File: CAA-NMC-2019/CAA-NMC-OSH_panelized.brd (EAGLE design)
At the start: 115.2 x 110.2 mm, 18 parts, among them IC1 ATTINY85-20SU, J1 M20-9980346

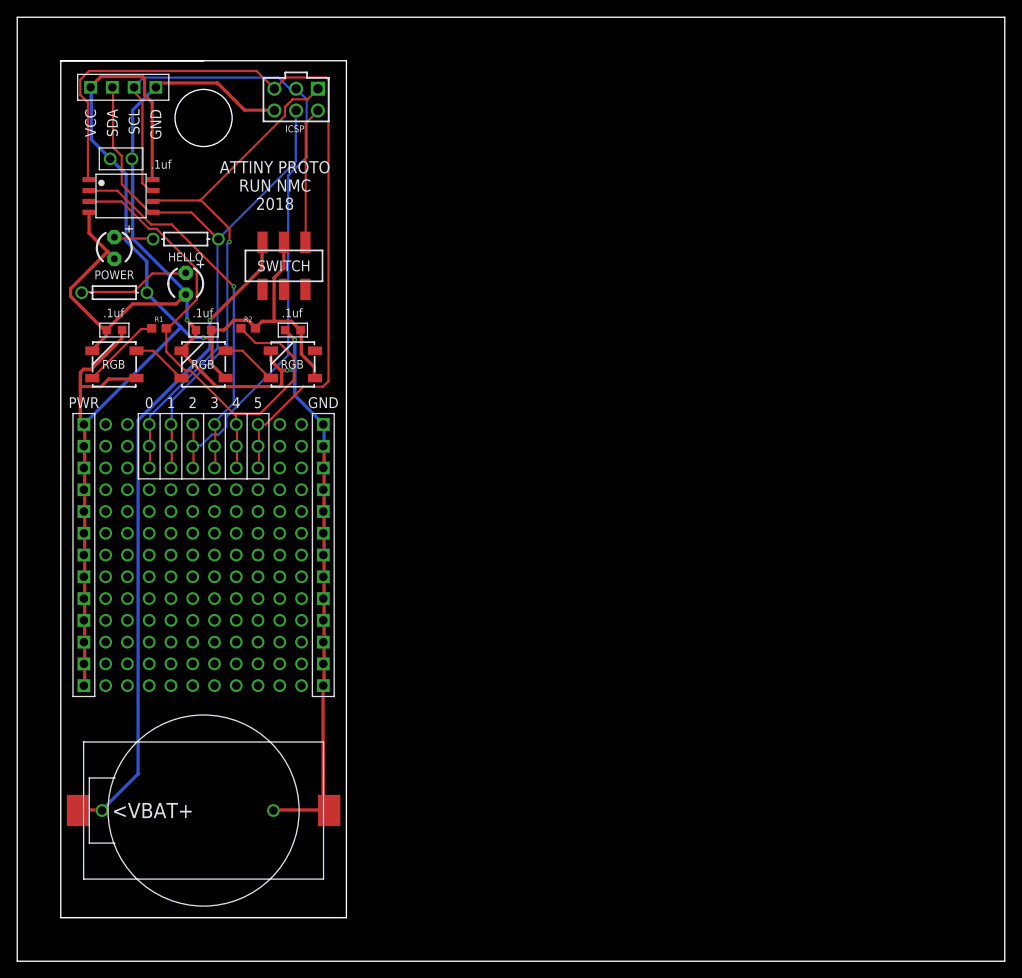
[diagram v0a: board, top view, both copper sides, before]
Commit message: Finalized file for OSH
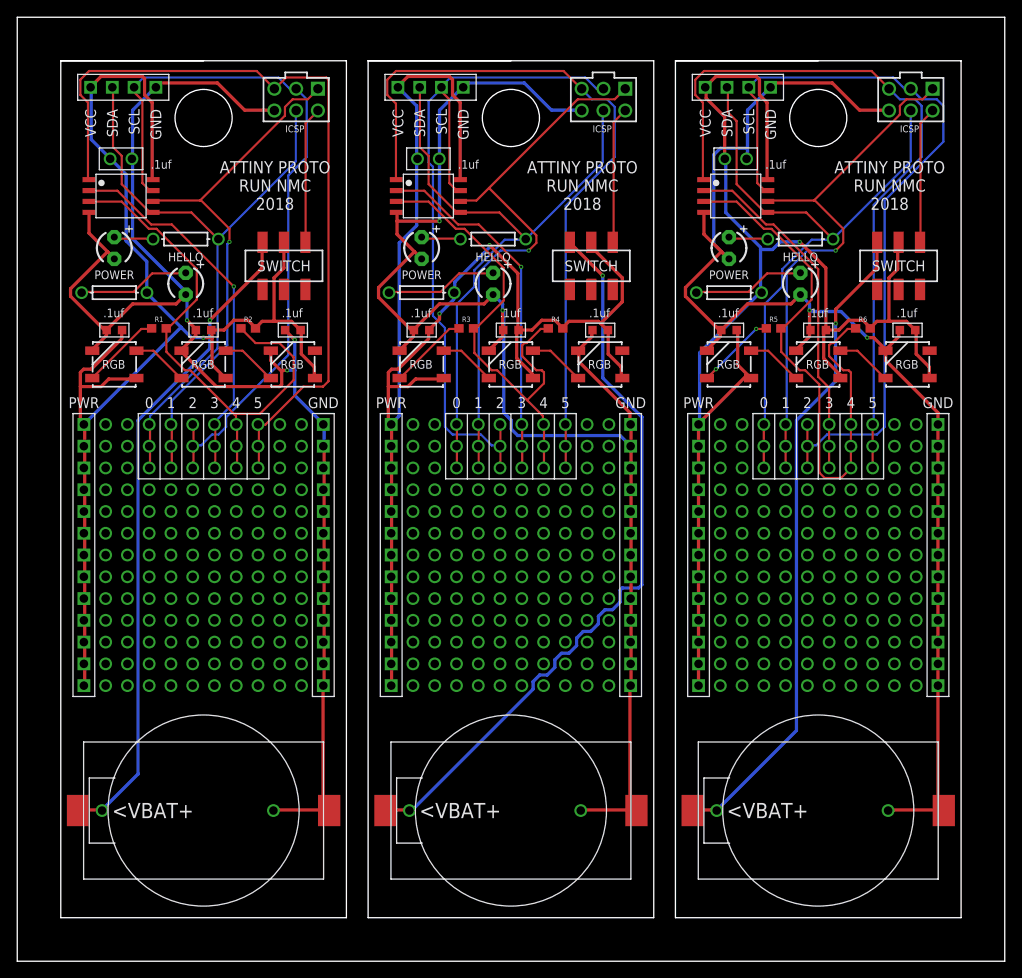
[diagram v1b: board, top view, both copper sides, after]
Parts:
- added D4, D5, D6, D7, D8, D9: WS2812B, BadgeParts:WS2812B
- added HELLO1, HELLO2, POWER1, POWER2: LED3MM, BadgeParts:LED3MM
- added IC2, IC3: ATTINY85-20SU, BadgeParts:SOT127P798X216-8N
- added J2, J3: M20-9980346, BadgeParts:HDRV6W64P254_2X3_762X508X868P
- added R3, R5: 470, SparkFun-Resistors:0603
- added R4, R6: 10k, SparkFun-Resistors:0603
- added U$10, U$19: PROTO, BadgeParts:PROTO
- added U$11, U$20: SMT-BATTERY-HOLDER, BadgeParts:SMT-CR-HOLDER
- added U$12, U$21: THRU-CR-HOLDER, BadgeParts:THRU-CR-HOLDER
- added U$13, U$22: I2C-PADS, BadgeParts:I2C-PADS
- added U$14, U$23: (no value), NickParts:OSHPARK_LOGOHEX
- added U$15, U$6: DECOUPLING_CAP, BadgeParts:DECOUPLING_CAP
- added U$16, U$17, U$7, U$8: RESISTOR, BadgeParts:AXIAL-0.3
- added U$18, U$9: SMT-SWITCH, BadgeParts:SMT-SWITCH
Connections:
- new net GND1: D4.CAP1, D4.GND, D5.CAP1, D5.GND, D6.CAP1, D6.GND, HELLO1.NEG, IC2.GND, J2.GND, POWER1.NEG, U$10.GND0, U$10.GND1, U$10.GND10, U$10.GND11, U$10.GND12, U$10.GND2, U$10.GND3, U$10.GND4, U$10.GND5, U$10.GND6, U$10.GND7, U$10.GND8, U$10.GND9, U$11.GND, U$12.GND, U$13.GND, U$6.P$1
- new net GND2: D7.CAP1, D7.GND, D8.CAP1, D8.GND, D9.CAP1, D9.GND, HELLO2.NEG, IC3.GND, J3.GND, POWER2.NEG, U$15.P$1, U$19.GND0, U$19.GND1, U$19.GND10, U$19.GND11, U$19.GND12, U$19.GND2, U$19.GND3, U$19.GND4, U$19.GND5, U$19.GND6, U$19.GND7, U$19.GND8, U$19.GND9, U$20.GND, U$21.GND, U$22.GND
- new net N$10: D4.DI, R3.1
- new net N$11: POWER2.POS, U$16.P$3
- new net N$12: HELLO2.POS, U$17.P$3
- new net N$13: D7.DO, D8.DI
- new net N$14: D8.DO, D9.DI
- new net N$15: D7.DI, R5.1
- new net N$6: POWER1.POS, U$7.P$3
- new net N$7: HELLO1.POS, U$8.P$3
- new net N$8: D4.DO, D5.DI
- new net N$9: D5.DO, D6.DI
- new net PB10: IC2.PB5, J2.5/RST, U$10.5A, U$10.5B, U$10.5C
- new net PB11: IC2.PB1, J2.1/MISO, U$10.1A, U$10.1B, U$10.1C
- new net PB12: IC3.PB0, J3.0/MOSI/SDA, U$17.P$4, U$19.0A, U$19.0B, U$19.0C, U$22.SDA
- new net PB13: IC3.PB3, U$19.3A, U$19.3B, U$19.3C
- new net PB14: IC3.PB4, R5.2, R6.1, U$19.4A, U$19.4B, U$19.4C
- new net PB15: IC3.PB2, J3.2/SCK/SCL, U$19.2A, U$19.2B, U$19.2C, U$22.SCL
- new net PB16: IC3.PB5, J3.5/RST, U$19.5A, U$19.5B, U$19.5C
- new net PB17: IC3.PB1, J3.1/MISO, U$19.1A, U$19.1B, U$19.1C
- new net PB6: IC2.PB0, J2.0/MOSI/SDA, U$10.0A, U$10.0B, U$10.0C, U$13.SDA, U$8.P$4
- new net PB7: IC2.PB3, U$10.3A, U$10.3B, U$10.3C
- new net PB8: IC2.PB4, R3.2, R4.1, U$10.4A, U$10.4B, U$10.4C
- new net PB9: IC2.PB2, J2.2/SCK/SCL, U$10.2A, U$10.2B, U$10.2C, U$13.SCL
- new net VBAT1: U$11.VBAT, U$12.VBAT, U$9.4
- new net VBAT2: U$18.4, U$20.VBAT, U$21.VBAT
- new net VCC1: D4.CAP2, D4.VCC, D5.CAP2, D5.VCC, D6.CAP2, D6.VCC, IC2.VCC, R4.2, U$10.PWR0, U$10.PWR1, U$10.PWR10, U$10.PWR11, U$10.PWR12, U$10.PWR2, U$10.PWR3, U$10.PWR4, U$10.PWR5, U$10.PWR6, U$10.PWR7, U$10.PWR8, U$10.PWR9, U$13.VCC, U$6.P$2, U$7.P$4, U$9.5
- new net VCC2: D7.CAP2, D7.VCC, D8.CAP2, D8.VCC, D9.CAP2, D9.VCC, IC3.VCC, R6.2, U$15.P$2, U$16.P$4, U$18.5, U$19.PWR0, U$19.PWR1, U$19.PWR10, U$19.PWR11, U$19.PWR12, U$19.PWR2, U$19.PWR3, U$19.PWR4, U$19.PWR5, U$19.PWR6, U$19.PWR7, U$19.PWR8, U$19.PWR9, U$22.VCC
- new net VUSB1: J2.VCC, U$9.6
- new net VUSB2: J3.VCC, U$18.6
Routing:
- net GND1: track 0.00 -> 174.3 mm, vias 0 -> 2
- net VCC1: track 0.00 -> 173.1 mm, vias 0 -> 2
- net VCC2: track 0.00 -> 160.9 mm, vias 0 -> 1
- net GND2: track 0.00 -> 160.5 mm, vias 0 -> 2
- net PB15: track 0.00 -> 93.1 mm
- net VBAT1: track 0.00 -> 87.2 mm, vias 0 -> 1
- net PB9: track 0.00 -> 86.8 mm
- net PB10: track 0.00 -> 85.4 mm
- net PB16: track 0.00 -> 85.2 mm
- net VBAT2: track 0.00 -> 76.9 mm, vias 0 -> 1
- net PB6: track 0.00 -> 76.1 mm
- net PB12: track 0.00 -> 76.0 mm
- net PB14: track 0.00 -> 67.6 mm
- net PB11: track 0.00 -> 64.4 mm, vias 0 -> 1
- net PB17: track 0.00 -> 62.7 mm, vias 0 -> 1
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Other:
- outline, holes or cut-outs redrawn
